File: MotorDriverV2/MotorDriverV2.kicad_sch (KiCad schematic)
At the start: 36 parts, among them IC1 DRV8871, IC2 DRV8871, IC3 ESP32-S3-WROOM-1U-N4, J1 Power, J2 Out_A, J3 Conn_01x02_Pin, J4 Conn_01x05_Pin, J5 Conn_01x05_Pin, J6 Out_B, J7 Conn_01x02_Pin, J8 USB_C, U1 USBLC6-2SC6

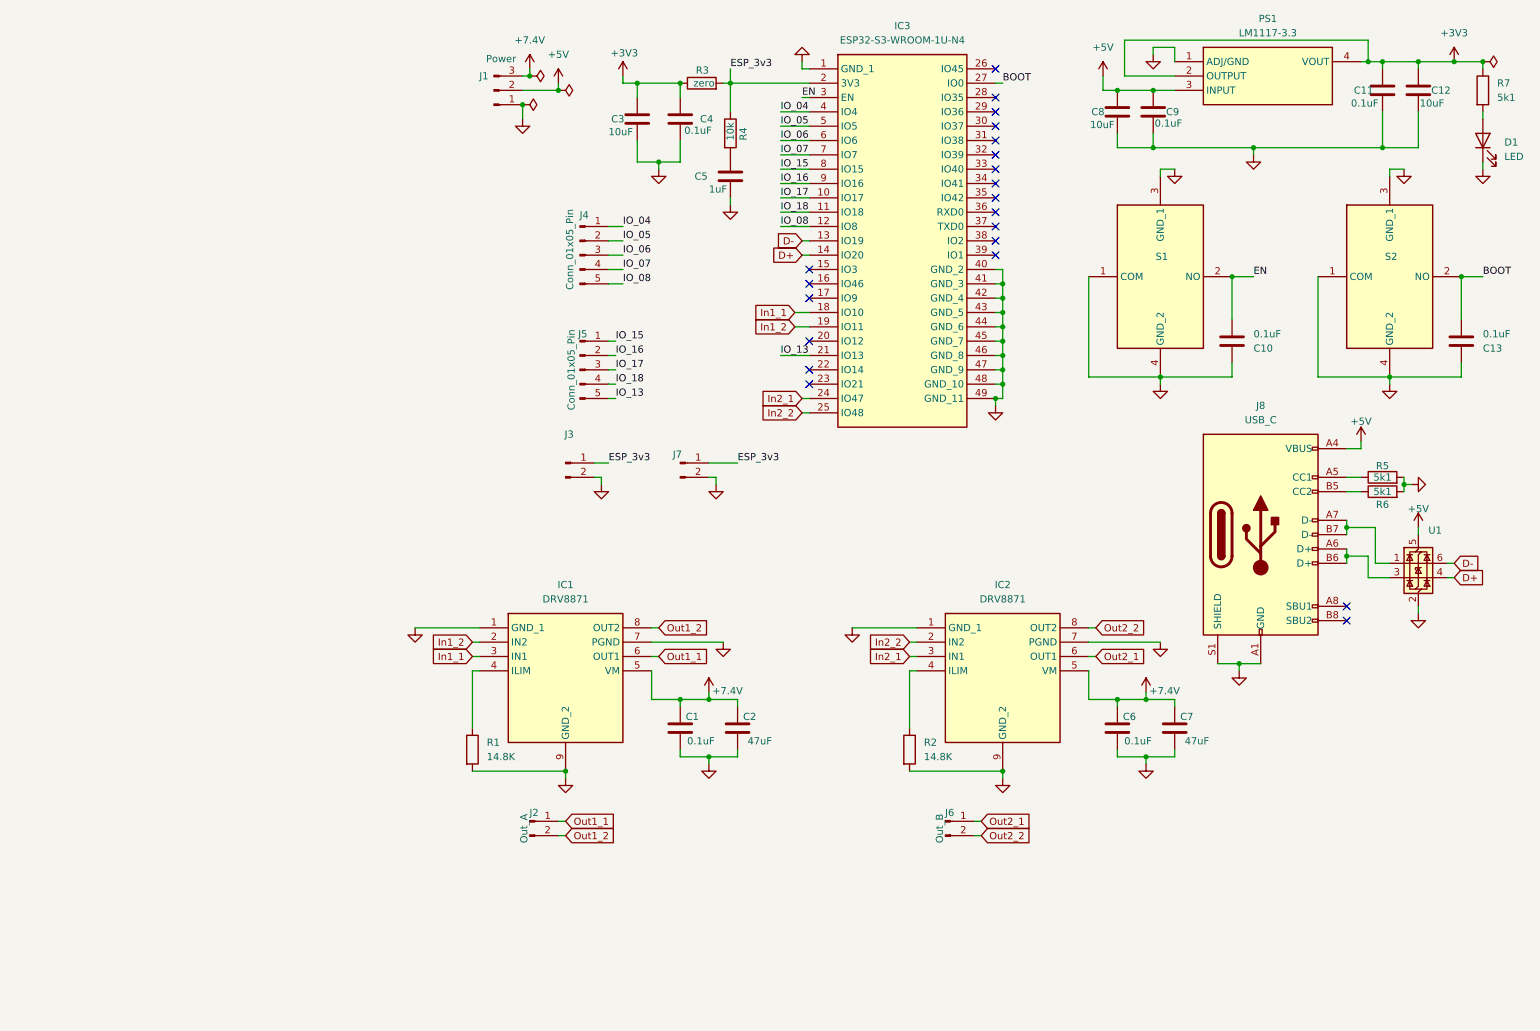
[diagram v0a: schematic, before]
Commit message: Completed PCB's
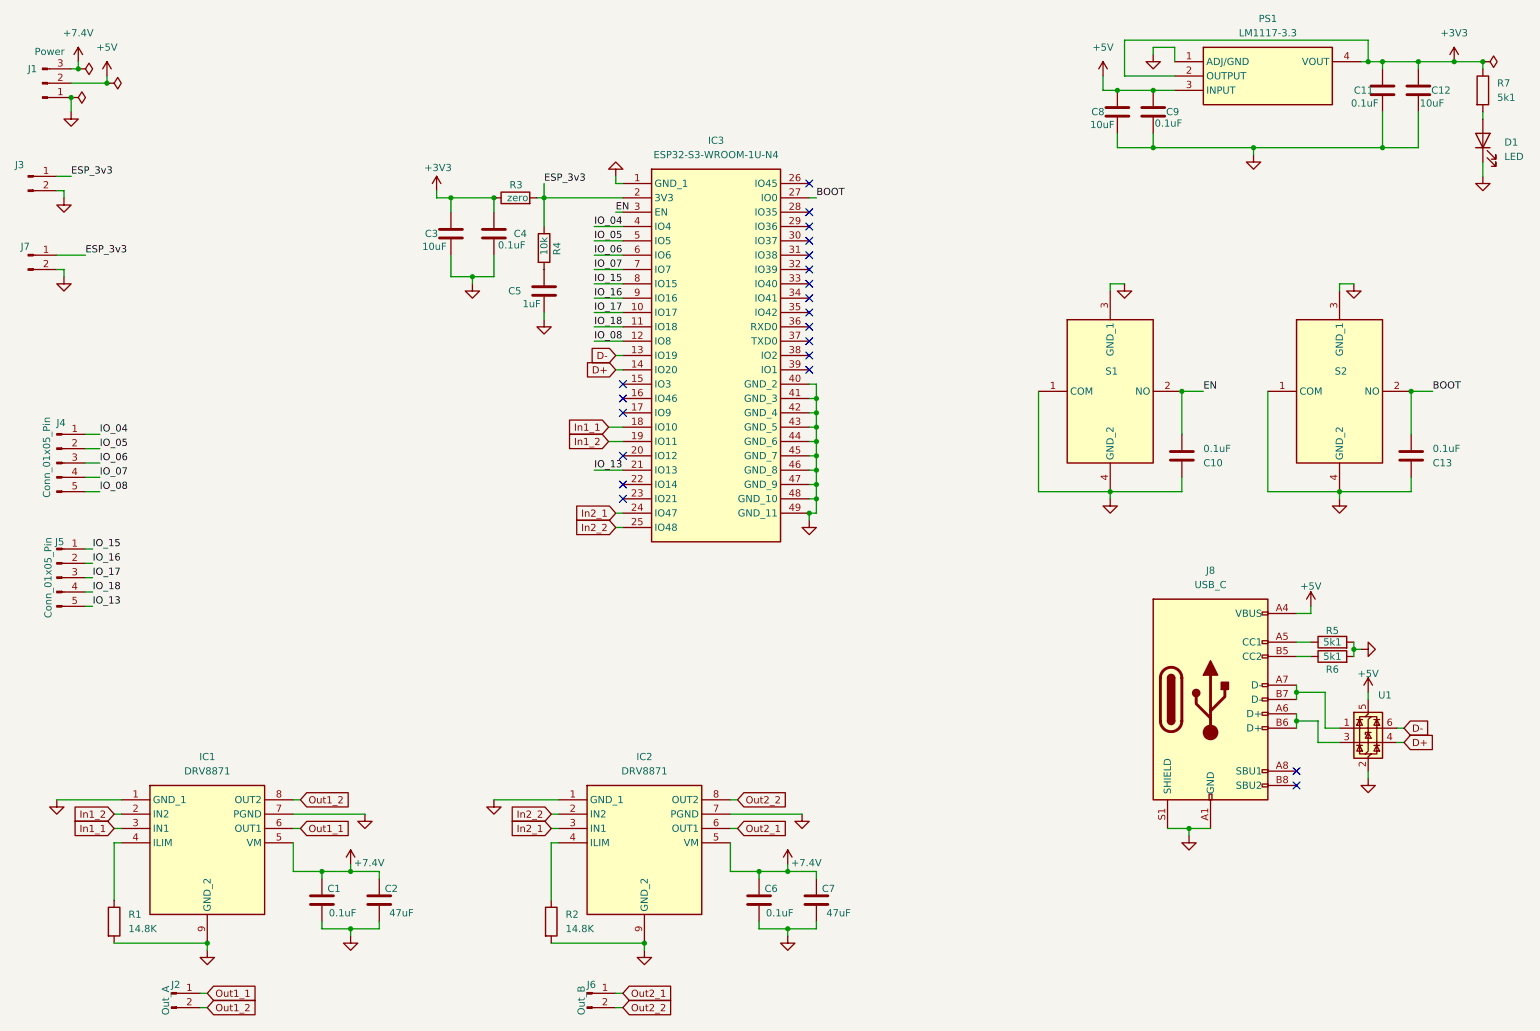
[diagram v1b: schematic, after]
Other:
- moved on the sheet: C1, C10, C13, C2, C3, C4, C5, C6, C7, IC1, IC2, IC3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
